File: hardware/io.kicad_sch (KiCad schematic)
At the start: 6 parts, among them J15 COM1, J16 COM2, J17 LPT, U20 68681

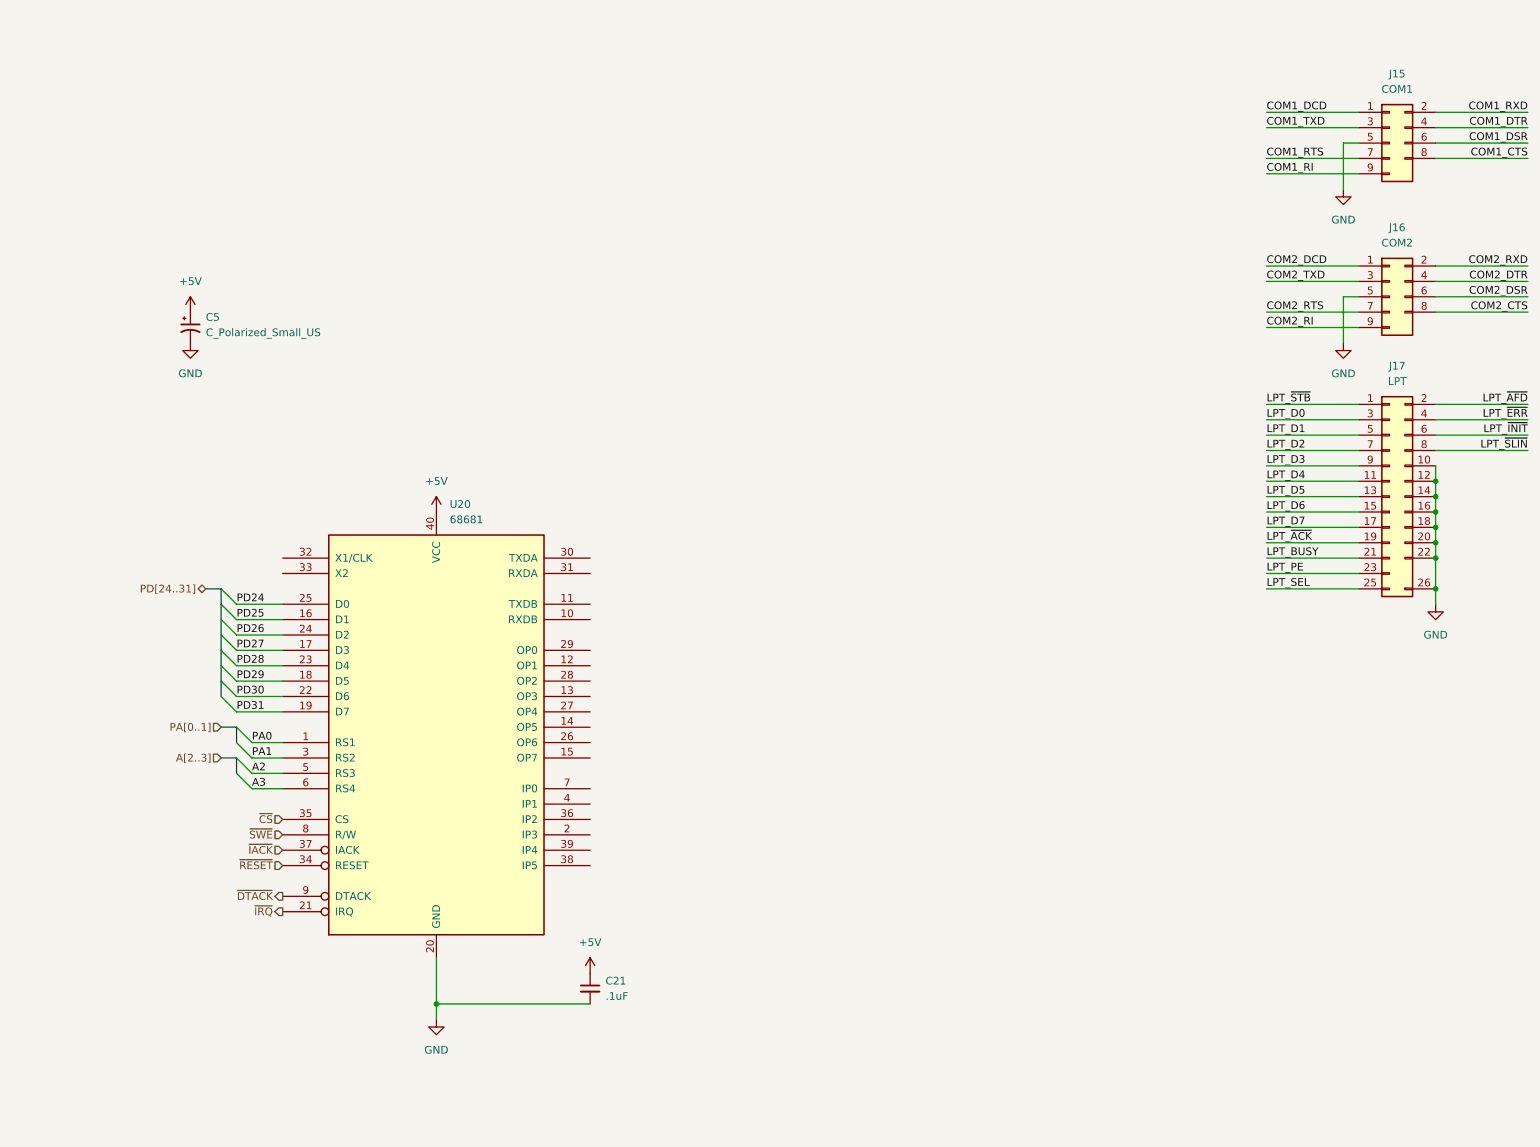
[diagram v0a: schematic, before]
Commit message: getting closer
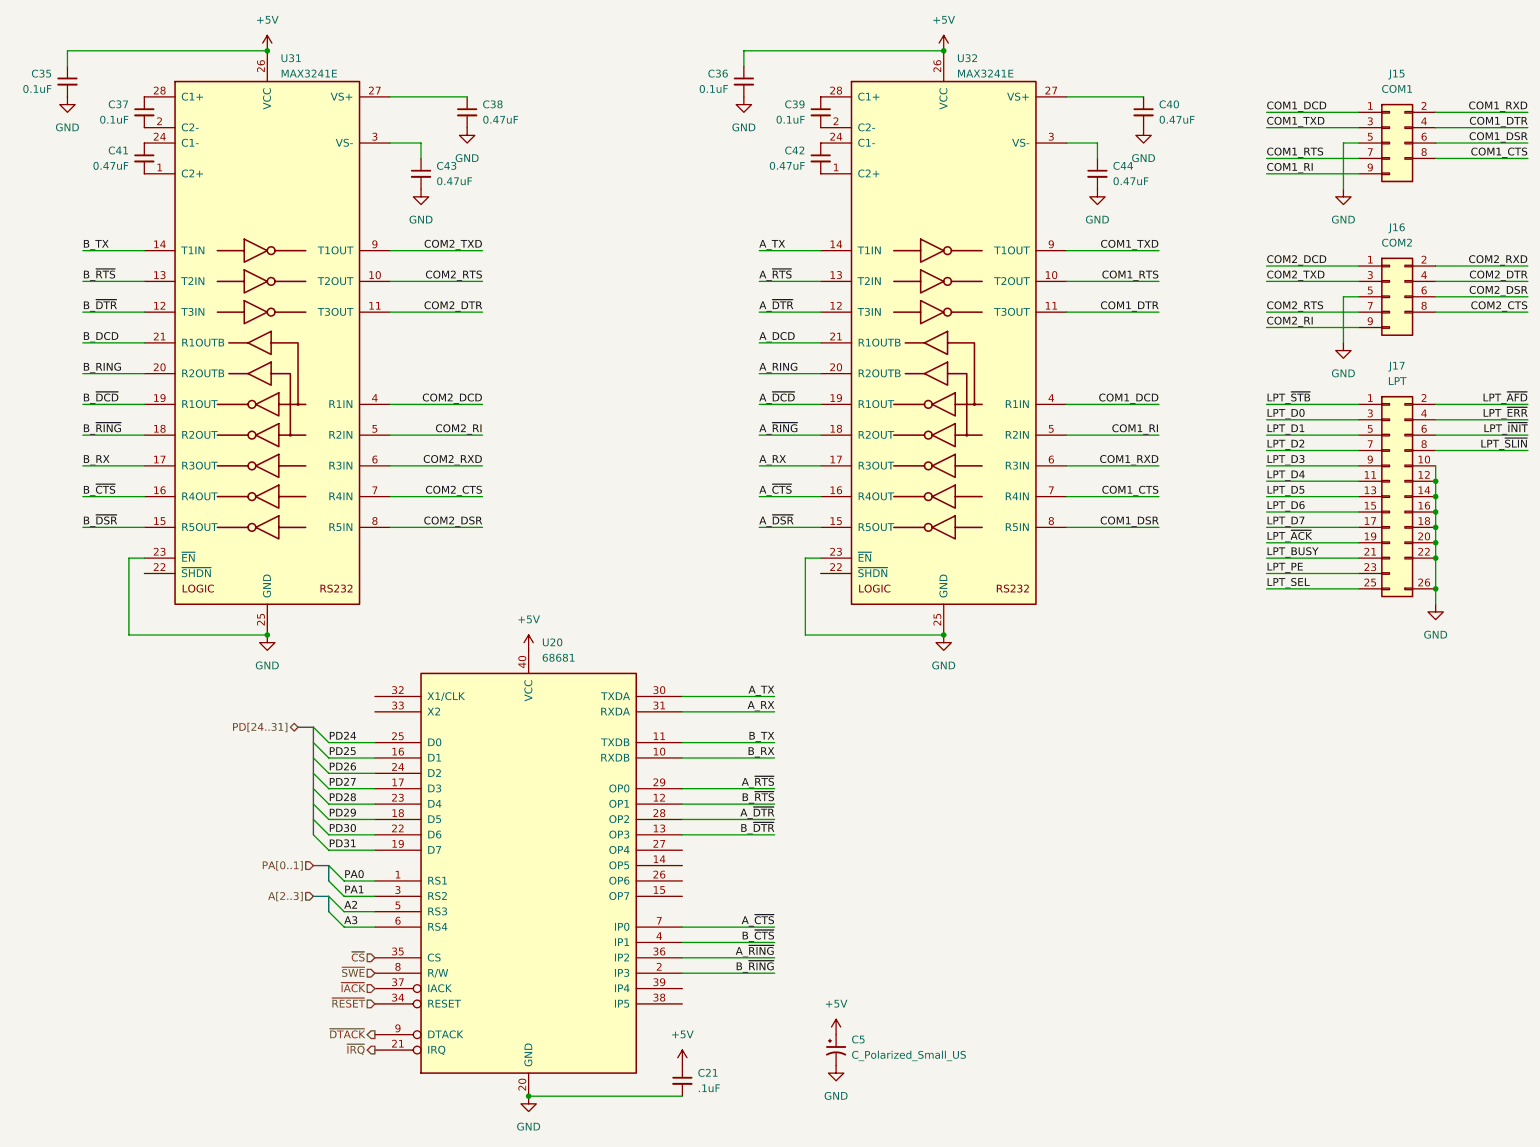
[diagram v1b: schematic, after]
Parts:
- added C35, C36, C37, C39: 0.1uF, symbol Device:C_Small
- added C38, C40, C41, C42, C43, C44: 0.47uF, symbol Device:C_Small
- added U31, U32: MAX3241E, symbol 68040:MAX3241E
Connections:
- net +5V: now also C35.1, C36.1, U31.26 (VCC), U32.26 (VCC)
- net COM1_CTS: now also U32.7 (R4IN)
- net COM1_DCD: now also U32.4 (R1IN)
- net COM1_DSR: now also U32.8 (R5IN)
- net COM1_DTR: now also U32.11 (T3OUT)
- net COM1_RI: now also U32.5 (R2IN)
- net COM1_RTS: now also U32.10 (T2OUT)
- net COM1_RXD: now also U32.6 (R3IN)
- net COM1_TXD: now also U32.9 (T1OUT)
- net COM2_CTS: now also U31.7 (R4IN)
- net COM2_DCD: now also U31.4 (R1IN)
- net COM2_DSR: now also U31.8 (R5IN)
- net COM2_DTR: now also U31.11 (T3OUT)
- net COM2_RI: now also U31.5 (R2IN)
- net COM2_RTS: now also U31.10 (T2OUT)
- net COM2_RXD: now also U31.6 (R3IN)
- net COM2_TXD: now also U31.9 (T1OUT)
- net GND: now also C35.2, C36.2, C38.2, C40.2, C43.2, C44.2, U31.23 (~{EN}), U31.25 (GND), U32.23 (~{EN}), U32.25 (GND)
- net B_RX: now reaches U20.10 (RXDB)
- net B_RX: now also U31.17 (R3OUT)
- net B_TX: now reaches U20.11 (TXDB)
- net B_TX: now also U31.14 (T1IN)
- net B_~{RTS}: now reaches U20.12 (OP1)
- net B_~{RTS}: now also U31.13 (T2IN)
- net B_~{DTR}: now reaches U20.13 (OP3)
- net B_~{DTR}: now also U31.12 (T3IN)
- net B_~{RING}: now reaches U20.2 (IP3)
- net B_~{RING}: now also U31.18 (R2OUT)
- net A_~{DTR}: now reaches U20.28 (OP2)
- net A_~{DTR}: now also U32.12 (T3IN)
- net A_~{RTS}: now reaches U20.29 (OP0)
- net A_~{RTS}: now also U32.13 (T2IN)
- net A_TX: now reaches U20.30 (TXDA)
- net A_TX: now also U32.14 (T1IN)
- net A_RX: now reaches U20.31 (RXDA)
- net A_RX: now also U32.17 (R3OUT)
- net A_~{RING}: now reaches U20.36 (IP2)
- net A_~{RING}: now also U32.18 (R2OUT)
- net B_~{CTS}: now reaches U20.4 (IP1)
- net B_~{CTS}: now also U31.16 (R4OUT)
- net A_~{CTS}: now reaches U20.7 (IP0)
- net A_~{CTS}: now also U32.16 (R4OUT)
- new net: C41.1, U31.24 (C1-)
- new net: C41.2, U31.1 (C2+)
- new net: C39.1, U32.28 (C1+)
- new net: C39.2, U32.2 (C2-)
- new net: C44.1, U32.3 (VS-)
- new net: C43.1, U31.3 (VS-)
- new net: C37.1, U31.28 (C1+)
- new net: C37.2, U31.2 (C2-)
- new net: C42.1, U32.24 (C1-)
- new net: C42.2, U32.1 (C2+)
- new net: C40.1, U32.27 (VS+)
- new net: C38.1, U31.27 (VS+)
- new net A_DCD: U32.21 (R1OUTB)
- new net A_RING: U32.20 (R2OUTB)
- new net A_~{DCD}: U32.19 (R1OUT)
- new net A_~{DSR}: U32.15 (R5OUT)
- new net B_DCD: U31.21 (R1OUTB)
- new net B_RING: U31.20 (R2OUTB)
- new net B_~{DCD}: U31.19 (R1OUT)
- new net B_~{DSR}: U31.15 (R5OUT)
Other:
- moved on the sheet: C21, C5, U20
